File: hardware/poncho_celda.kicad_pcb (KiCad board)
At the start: 2 copper layers, 20 parts, among them U1 AD620, U2 REF1004-2.5, U3 ADS1113/15

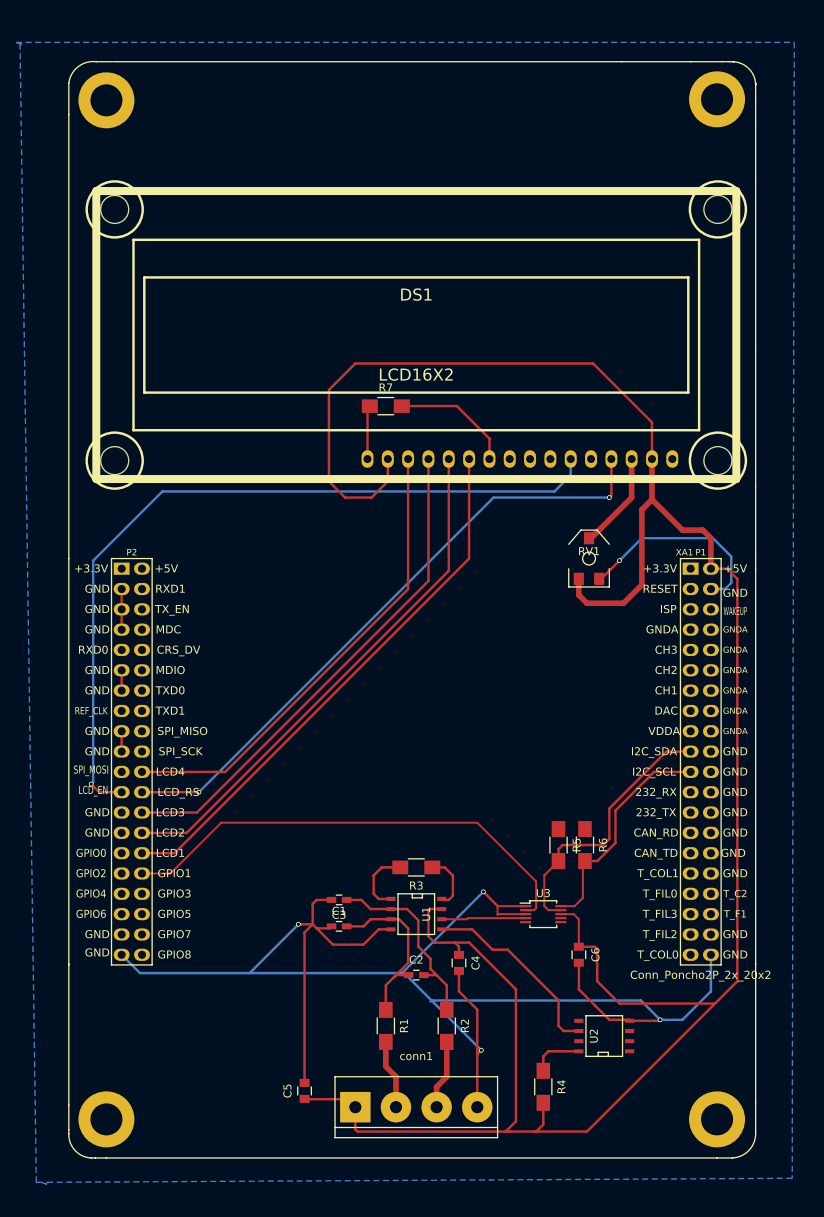
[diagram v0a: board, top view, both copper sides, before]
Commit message: Primera version de de diseño de PCB, terminado.
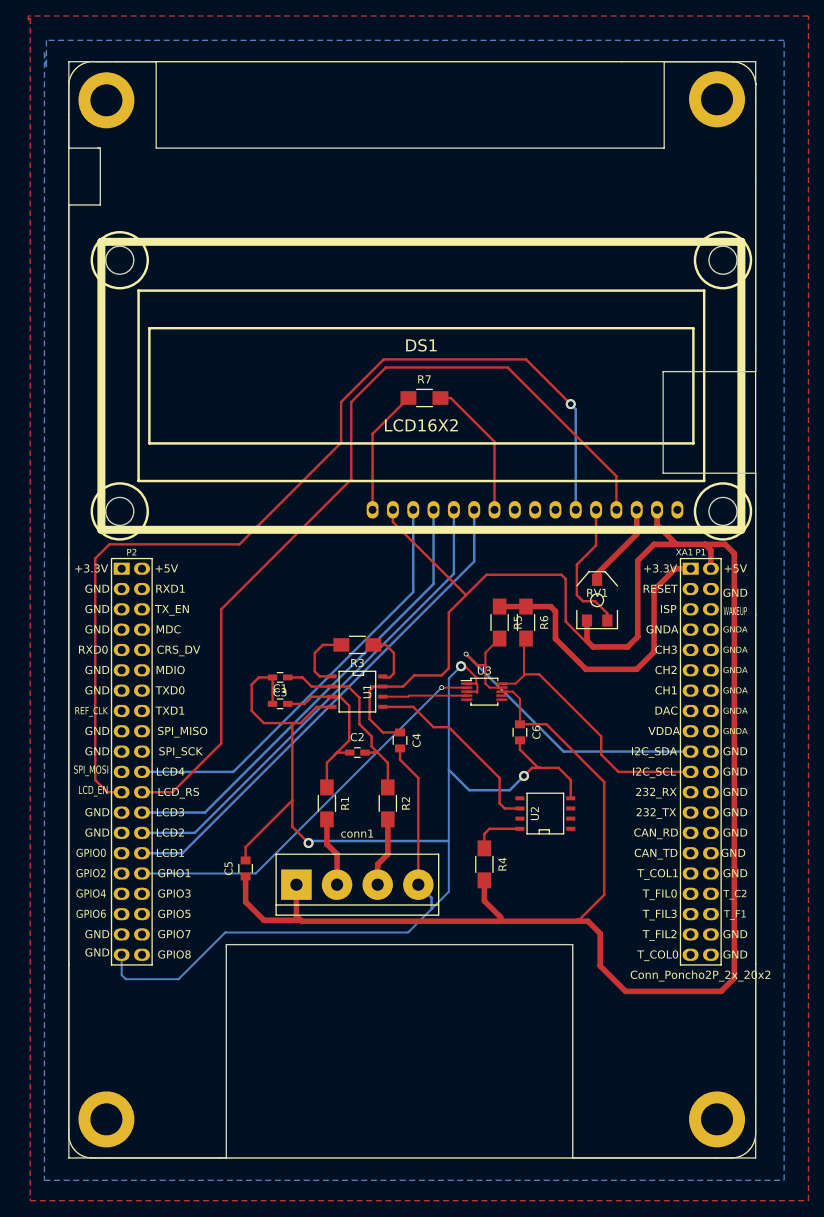
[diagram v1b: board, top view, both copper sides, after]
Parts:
- moved C3 28.8 mm to (103.6, 115.2)
- moved R4 28.8 mm to (129.2, 138.6)
- moved U2 28.8 mm to (136.8, 132.2)
- moved C6 28.8 mm to (133.6, 122.0)
- moved C1 28.8 mm to (103.6, 118.5)
- moved C2 28.8 mm to (113.3, 124.6)
- moved C4 28.8 mm to (118.6, 123.1)
- moved R5 28.8 mm to (131.1, 108.3)
- moved U1 28.8 mm to (113.3, 117.0)
- moved U3 28.8 mm to (129.2, 117.0)
- moved R6 28.8 mm to (134.4, 108.3)
- moved C5 28.8 mm to (99.3, 139.1)
- moved R1 28.8 mm to (109.5, 130.9)
- moved R2 28.8 mm to (117.1, 130.9)
- moved R3 28.8 mm to (113.3, 111.1)
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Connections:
- R5 pad 1: +3.3V -> +3V3
- R6 pad 1: +3.3V -> +3V3
- XA1 pad 1: Net-(XA1-Pad1) -> +3V3
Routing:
- net +3V3: track 0.00 -> 38.9 mm
- net /lcd/RS: track 78.6 -> 106.6 mm, vias 2 -> 0
- net +5V: track 304.4 -> 281.4 mm
- net GND: track 251.9 -> 230.0 mm, vias 5 -> 3
- net /lcd/Ena: track 98.4 -> 120.1 mm
- net /ADC/sda: track 33.9 -> 44.8 mm, vias 0 -> 1
- net /ADC/alert: track 59.7 -> 50.2 mm, vias 0 -> 1
- net Net-(DS1-Pad16): track 6.73 -> 15.8 mm
- net /ADC/scl: track 28.1 -> 35.1 mm
- net /lcd/D2: track 65.9 -> 60.4 mm
- net /lcd/D1: track 68.6 -> 63.1 mm
- net /lcd/D4: track 59.0 -> 53.5 mm
- net /lcd/D3: track 63.0 -> 57.5 mm
- net Net-(DS1-Pad3): track 12.3 -> 10.8 mm
- added copper zone on F.Cu, net +5V
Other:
- board outline added: 85.9 x 137 mm
